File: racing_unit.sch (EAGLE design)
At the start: 45 parts, among them IC1 7805, IC2 7805, IC3 7805, IC4 7805, Q1 MJE2955, Q2 MJE2955, Q3 MJE2955, Q4 MJE2955

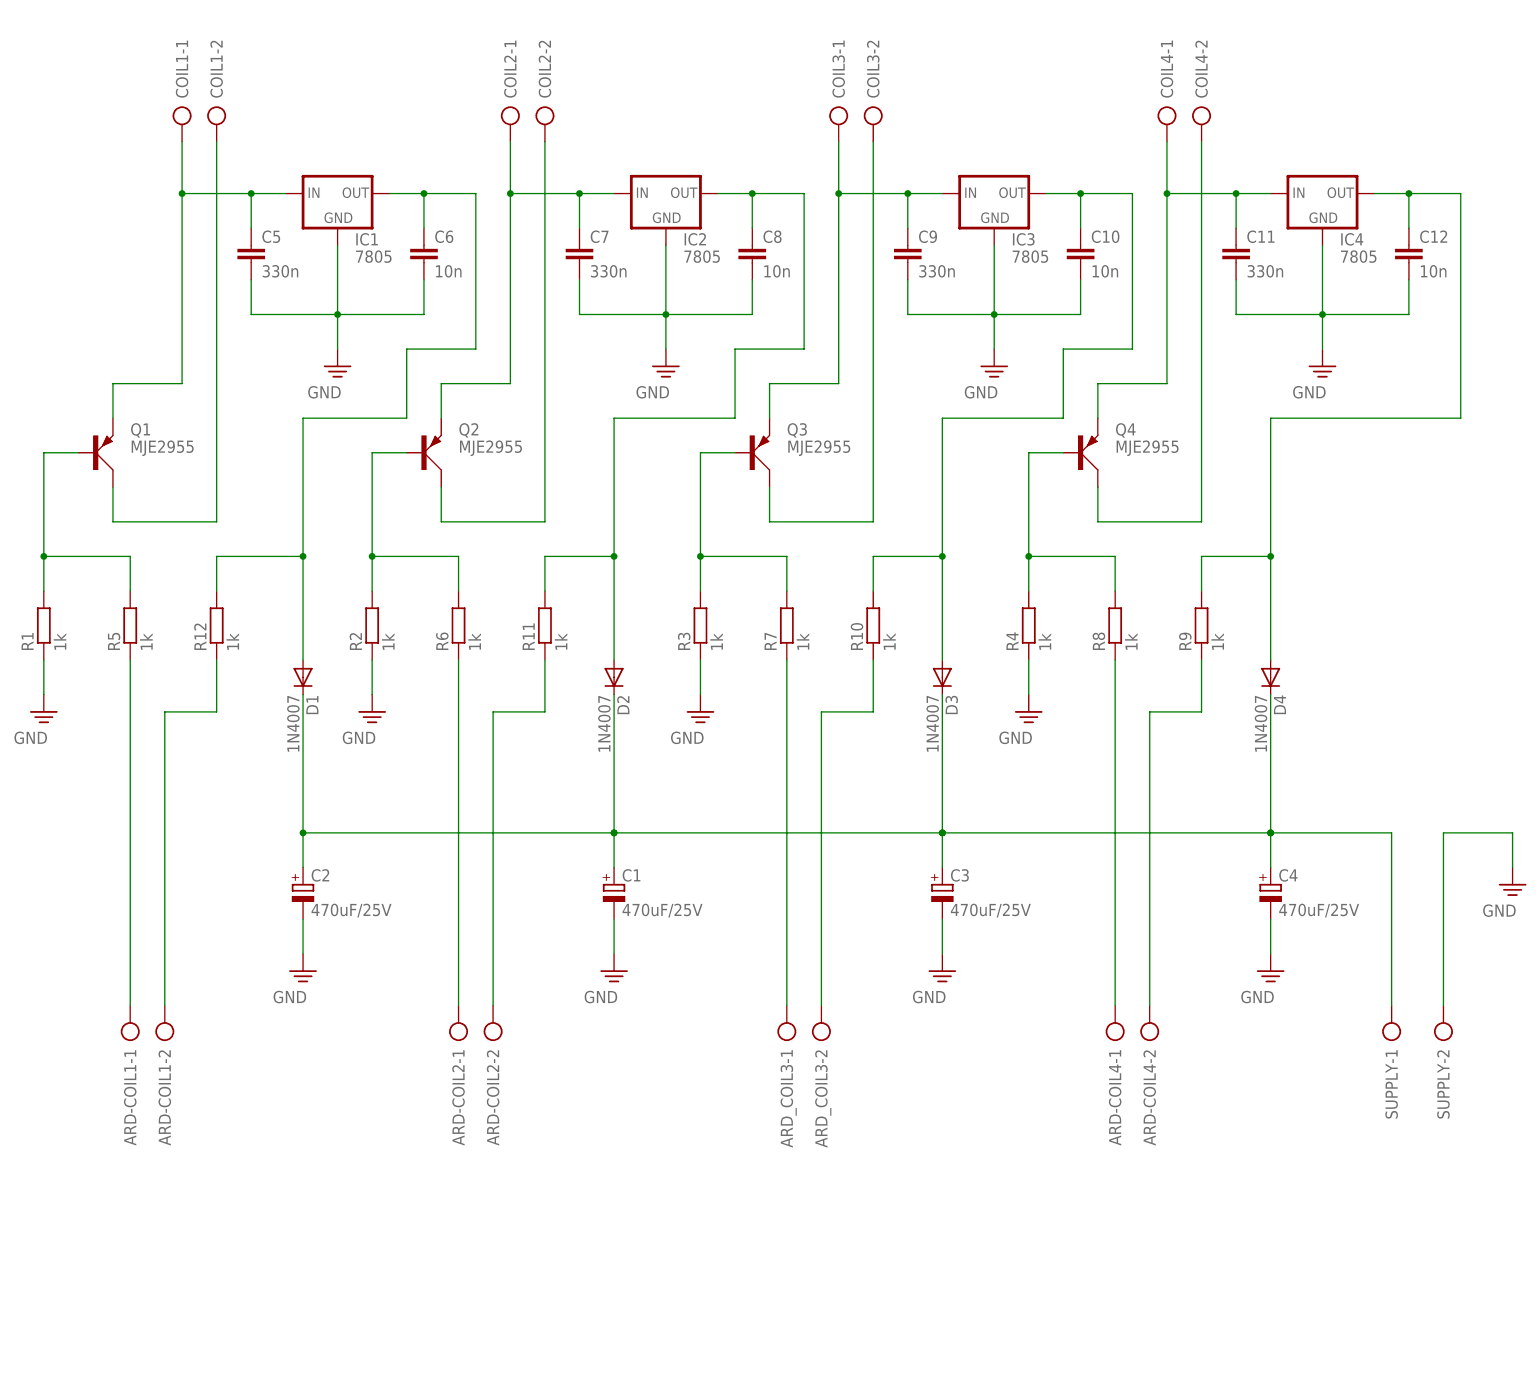
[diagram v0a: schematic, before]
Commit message: updated schematic
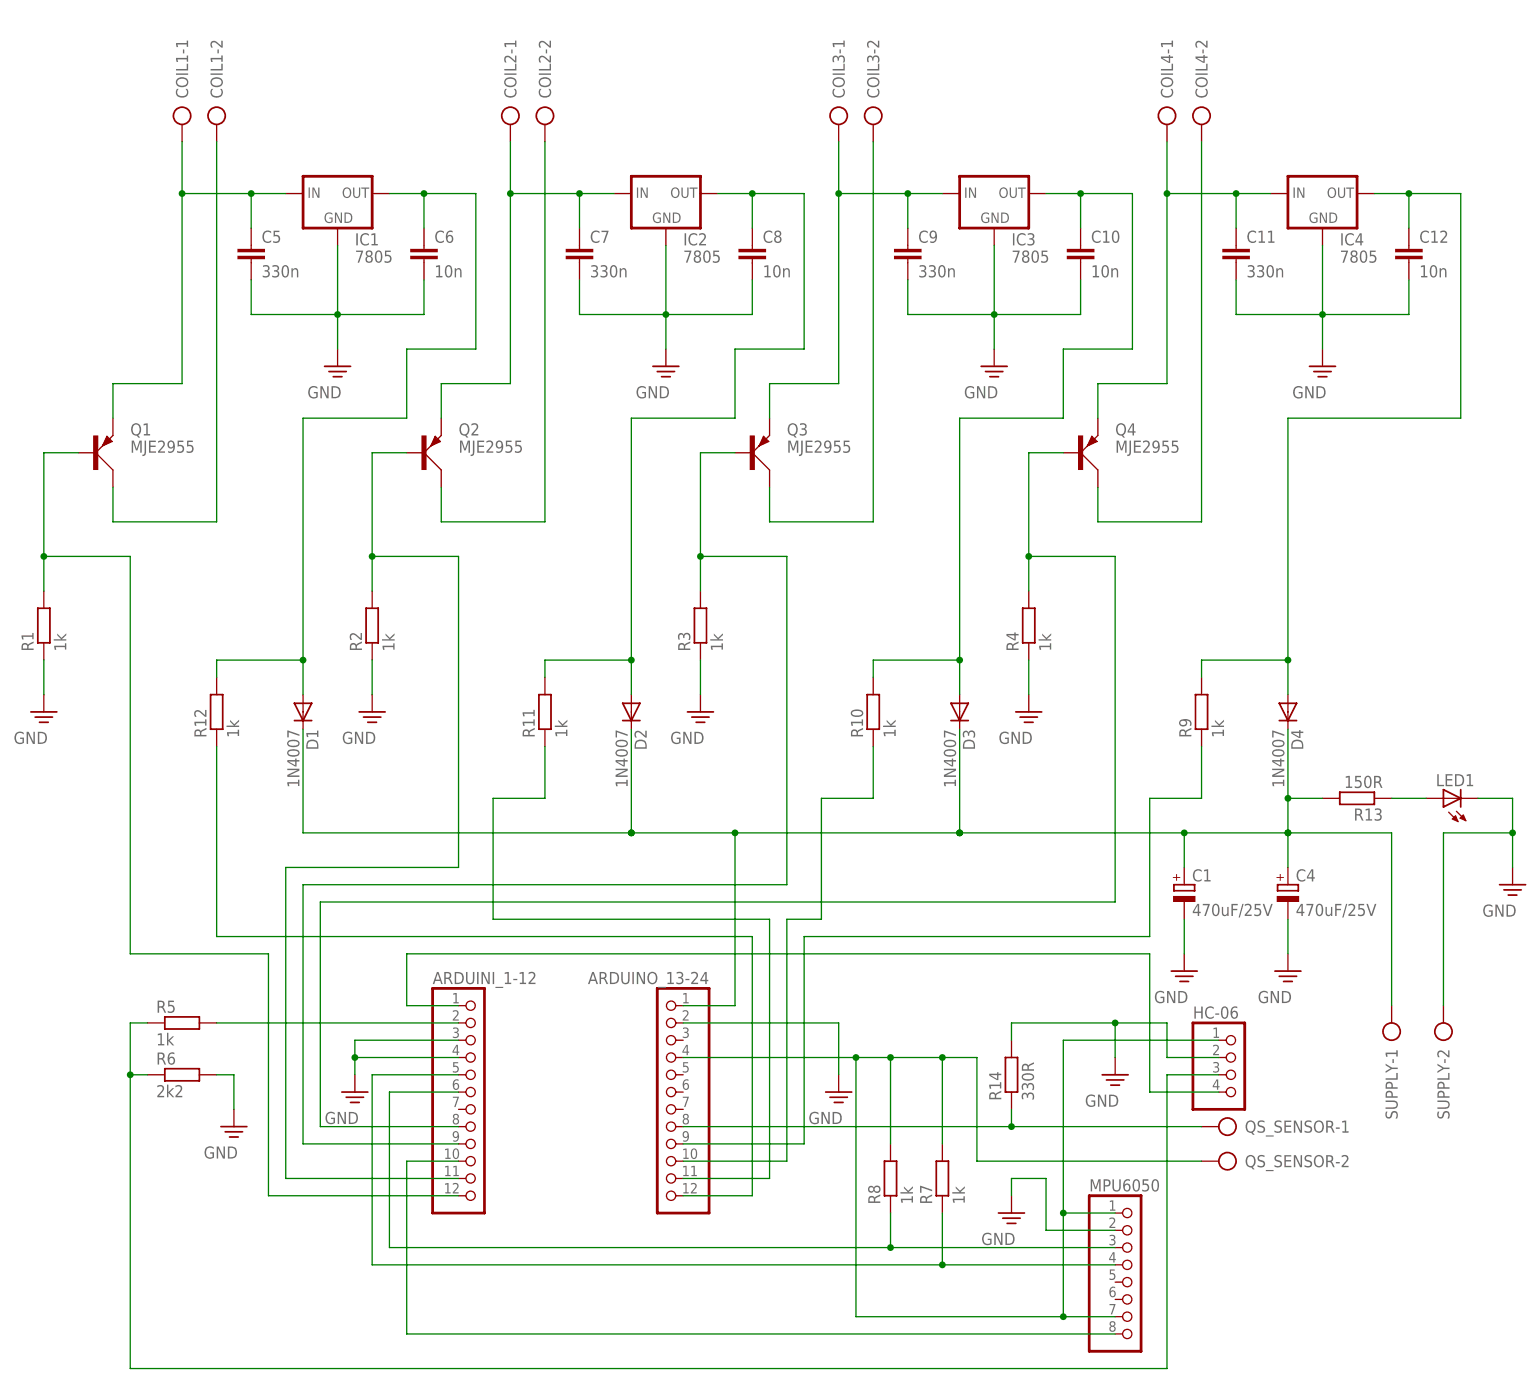
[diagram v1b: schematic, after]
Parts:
- removed ARD-COIL1, ARD-COIL2, ARD-COIL4, ARD_COIL3: (no value), con-ptr500:AK500/2
- removed C2, C3: 470uF/25V, rcl:CPOL-EUE3.5-8
- added ARDUINI_1-12, ARDUINO_13-24: (no value), pinhead:PINHD-1X12
- added HC-06: (no value), pinhead:PINHD-1X4
- added LED1: (no value), led:LED3MM
- added MPU6050: (no value), pinhead:PINHD-1X8
- added QS_SENSOR: (no value), con-ptr500:AK500/2
- added R13: 150R, resistor:R-EU_0204/5
- added R14: 330R, resistor:R-EU_0204/5
- R6: value 1k -> 2k2
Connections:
- new net N$13: LED1.A, R13.1
- new net N$27: ARDUINI_1-12.6, MPU6050.3, R8.1
- new net N$28: ARDUINI_1-12.2, R5.2
- new net N$30: ARDUINO_13-24.1, C1.+, C4.+, D1.C, D2.C, D3.C, D4.C, R13.2, SUPPLY-1.KL
- new net N$32: HC-06.3, R5.1, R6.1
- net N$16: now also ARDUINO_13-24.8, QS_SENSOR-1.KL, R14.1; no longer ARD-COIL2-1.KL, R6.1
- net N$18: now also ARDUINI_1-12.5, MPU6050.4, R7.1; no longer C1.+, C2.+, C3.+, C4.+, D1.C, D2.C, D3.C, D4.C, SUPPLY-1.KL
- net N$19: now also ARDUINI_1-12.9; no longer R7.2
- net N$20: now also ARDUINI_1-12.10, MPU6050.8; no longer ARD_COIL3-1.KL, R7.1
- net N$22: now also ARDUINI_1-12.1, HC-06.4; no longer ARD-COIL4-1.KL, R8.1
- net N$23: now also ARDUINO_13-24.12; no longer ARD-COIL1-2.KL
- net N$24: now also ARDUINO_13-24.11; no longer ARD-COIL2-2.KL
- net N$25: now also ARDUINO_13-24.10; no longer ARD_COIL3-2.KL
- net N$26: now also ARDUINO_13-24.9; no longer ARD-COIL4-2.KL
- net N$5: now also ARDUINO_13-24.4, HC-06.1, MPU6050.1, MPU6050.7, QS_SENSOR-2.KL, R7.2, R8.2; no longer ARD-COIL1-1.KL, R5.1
- net N$6: now also ARDUINI_1-12.12; no longer R5.2
- net N$7: now also ARDUINI_1-12.11; no longer R6.2
- net N$8: now also ARDUINI_1-12.8; no longer R8.2
- net PE: now also ARDUINI_1-12.3, ARDUINI_1-12.4, ARDUINO_13-24.2, HC-06.2, LED1.C, MPU6050.2, R14.2, R6.2; no longer C2.-, C3.-
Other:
- moved on the sheet: C1, C4, D1, D2, D3, D4, R10, R11, R12, R5, R6, R7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
